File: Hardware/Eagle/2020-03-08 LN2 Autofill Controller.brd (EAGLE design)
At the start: 114.3 x 95.2 mm, 28 parts, among them SW1 Omron B3J-2100, SW2 Omron B3J-2100, SW3 Omron B3J-2100, SW4 Omron B3J-2100, U1 MC14490DWG, U3 ISO7421DR

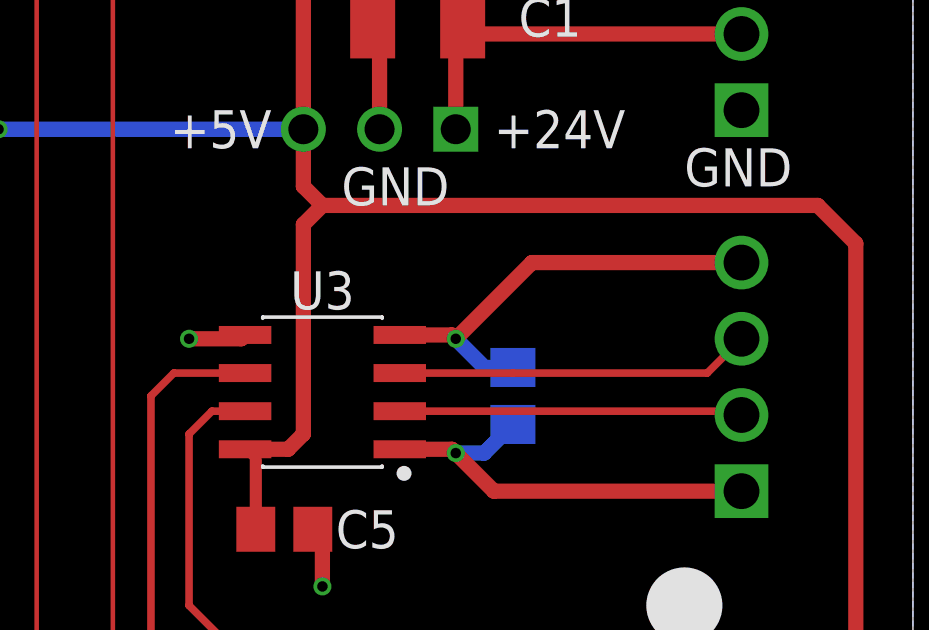
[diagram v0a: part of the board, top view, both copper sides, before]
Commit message: Save minor changes?
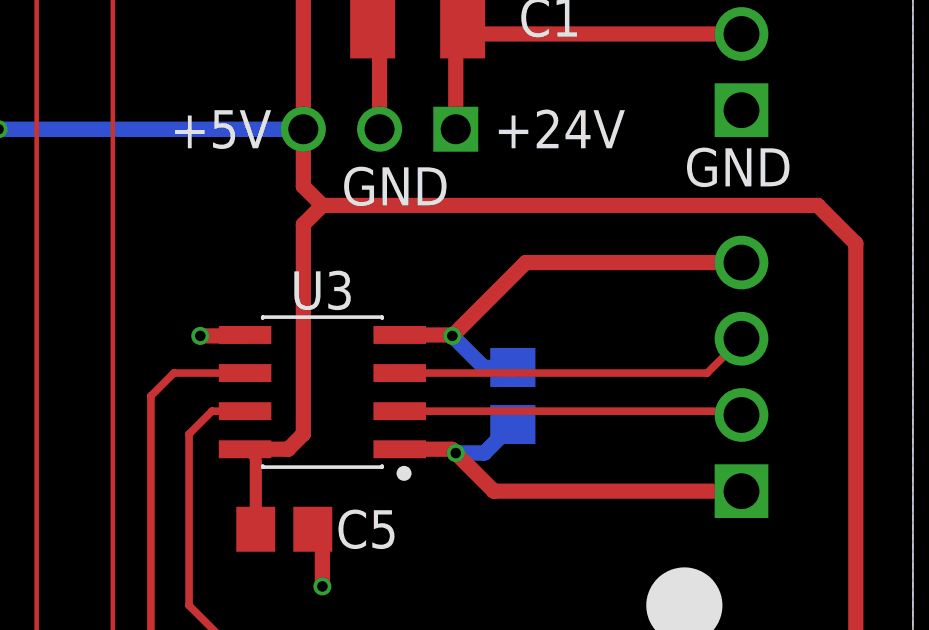
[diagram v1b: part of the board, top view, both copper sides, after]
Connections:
- net N$4 renamed /RES
